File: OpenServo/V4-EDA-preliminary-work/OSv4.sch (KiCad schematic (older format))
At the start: 0 parts

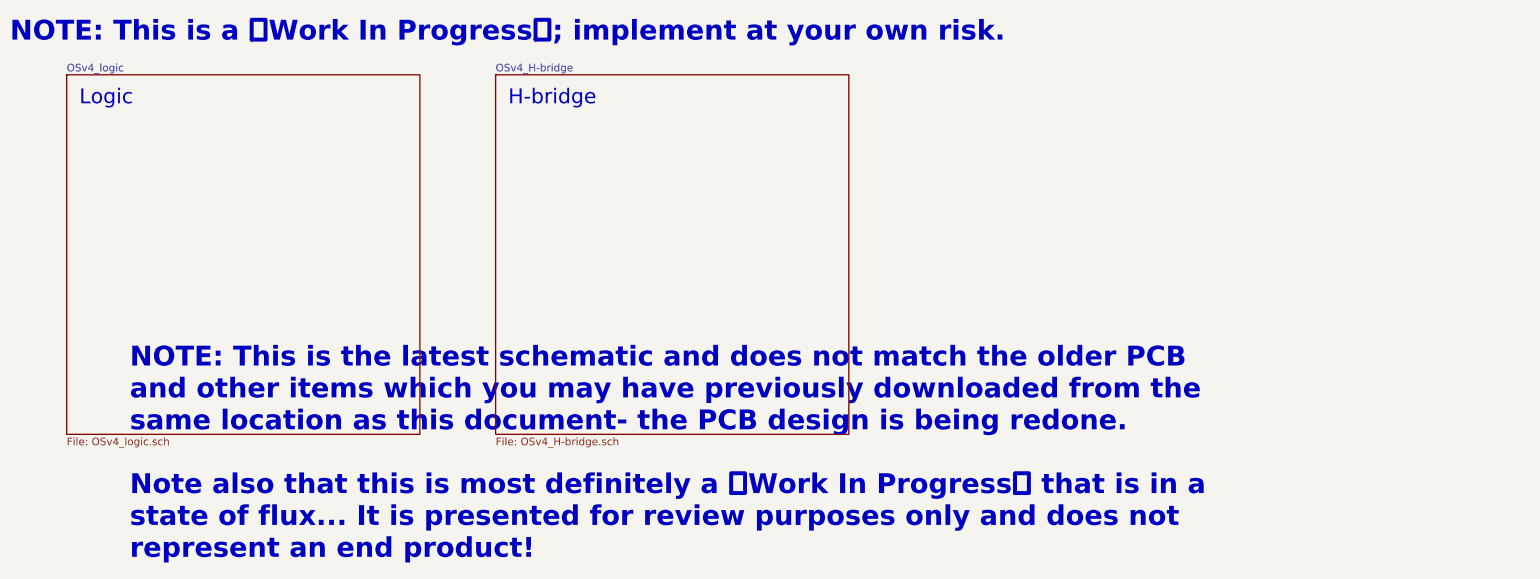
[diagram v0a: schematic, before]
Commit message: no message
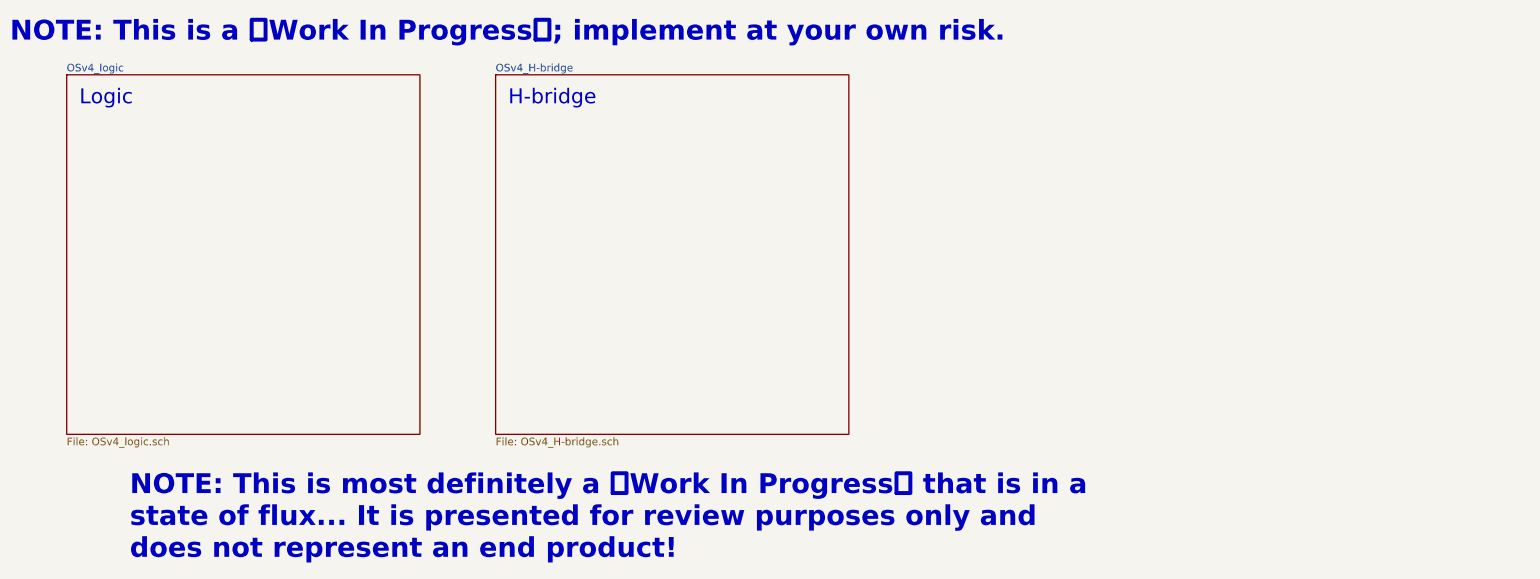
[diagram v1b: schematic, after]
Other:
- note added: "NOTE: This is most definitely a Work In Progress that is in a\nstate of flux... It is presented for review purposes only and\ndoes not represent an end product!"
- note removed: "NOTE: This is the latest schematic and does not match the older PCB\nand other items which you may have previously downloaded from the\nsame location as this document- the PCB design is being redone.\n\nNote also that this is most definitely a Work In Progress that is in a\nstate of flux... It is presented for review purposes only and does not\nrepresent an end product!"
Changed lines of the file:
@@
-EESchema Schematic File Version 2  date 08/05/2010 23:44:42
+EESchema Schematic File Version 2  date 11/05/2010 23:49:02
 LIBS:power
 LIBS:device
@@
 Sheet 1 3
 Title "OpenServo v4 preliminary work-up, © OpenServo project 2010"
-Date "8 may 2010"
+Date "11 may 2010"
 Rev ""
 Comp ""
@@
 $EndDescr
 Text Notes 1550 4900 0    157  ~ 31
-NOTE: This is the latest schematic and does not match the older PCB\nand other items which you may have previously downloaded from the\nsame location as this document- the PCB design is being redone.\n\nNote also that this is most definitely a Work In Progress that is in a\nstate of flux... It is presented for review purposes only and does not\nrepresent an end product!
+NOTE: This is most definitely a Work In Progress that is in a\nstate of flux... It is presented for review purposes only and\ndoes not represent an end product!
 Text Notes 600  800  0    157  ~ 31
 NOTE: This is a Work In Progress; implement at your own risk.
